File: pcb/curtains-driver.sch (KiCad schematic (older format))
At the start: 40 parts, among them J1 Barrel_Jack, J2 USB_B_Micro, J3 Motor, Q1 S8050, Q2 S8050, SW1 Reed_NC, SW2 Reed_NC, SW3 UP, SW4 DOWN, SW5 FLASH, SW6 RESET, U1 ESP-12F, U2 LM1117-3.3, U3 ULN2003, U4 CH340G, Y1 HC-49

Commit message: Update PCB
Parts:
- added R14: 10K, Resistor_SMD:R_0805_2012Metric_Pad1.15x1.40mm_HandSolder, symbol Device:R
- J1: symbol Connector:Barrel_Jack -> curtains-driver-rescue:Barrel_Jack-Connector
- SW5, SW6: footprint Button_Switch_SMD:SW_SPST_B3U-1000P -> Button_Switch_SMD:SW_SPST_TL3342
- U3: value ULN2003 -> ULN2003A
- Y1: footprint Crystal:Crystal_SMD_HC49-SD_HandSoldering -> Crystal:Crystal_SMD_SeikoEpson_FA238V-4Pin_3.2x2.5mm_HandSoldering; symbol Device:Crystal -> Device:Crystal_GND24_Small
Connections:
- wire segments 156 -> 159
- no-connect marks 20 -> 22
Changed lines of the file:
@@
 EESchema Schematic File Version 4
 LIBS:curtains-driver-cache
-EELAYER 26 0
+EELAYER 29 0
 EELAYER END
 $Descr A4 11693 8268
@@
 $EndComp
 $Comp
-L Connector:Barrel_Jack J1
+L curtains-driver-rescue:Barrel_Jack-Connector J1
 U 1 1 5C0D7D27
 P 5150 1750
@@
 P 9850 4250
 F 0 "U3" H 9850 4917 50  0000 C CNN
-F 1 "ULN2003" H 9850 4826 50  0000 C CNN
+F 1 "ULN2003A" H 9850 4826 50  0000 C CNN
 F 2 "Package_SO:SOIC-16W_5.3x10.2mm_P1.27mm" H 9900 3700 50  0001 L CNN
 F 3 "http://www.ti.com/lit/ds/symlink/uln2003a.pdf" H 9950 4050 50  0001 C CNN
@@
 F 0 "SW5" H 9500 5400 50  0000 L CNN
 F 1 "FLASH" H 9500 5300 50  0000 L CNN
-F 2 "Button_Switch_SMD:SW_SPST_B3U-1000P" H 9600 5150 50  0001 C CNN
+F 2 "Button_Switch_SMD:SW_SPST_TL3342" H 9600 5150 50  0001 C CNN
 F 3 "" H 9600 5150 50  0001 C CNN
 	1    9600 5150
@@
 	8700 5050 8700 5800
 Wire Wire Line
-	8950 3800 8950 4350
-Wire Wire Line
-	9050 3800 9050 4450
+	9050 3800 9050 4350
+Wire Wire Line
+	9150 3800 9150 4450
 $Comp
 L Switch:SW_SPST SW6
@@
 F 0 "SW6" H 6200 4000 50  0000 L CNN
 F 1 "RESET" H 6200 3900 50  0000 L CNN
-F 2 "Button_Switch_SMD:SW_SPST_B3U-1000P" H 6250 3750 50  0001 C CNN
+F 2 "Button_Switch_SMD:SW_SPST_TL3342" H 6250 3750 50  0001 C CNN
 F 3 "" H 6250 3750 50  0001 C CNN
 	1    6250 3750
@@
 	8650 4550 9450 4550
 Wire Wire Line
-	8650 4450 9050 4450
-Wire Wire Line
-	9050 4450 9450 4450
-Connection ~ 9050 4450
-Wire Wire Line
-	8650 4350 8950 4350
-Wire Wire Line
-	8950 4350 9450 4350
-Connection ~ 8950 4350
+	8650 4450 9150 4450
+Wire Wire Line
+	9150 4450 9450 4450
+Connection ~ 9150 4450
+Wire Wire Line
+	8650 4350 8800 4350
+Wire Wire Line
+	9050 4350 9450 4350
+Connection ~ 9050 4350
 Wire Wire Line
 	9850 5150 9850 4850
@@
 	1    0    0    -1
 $EndComp
-Text GLabel 8950 3800 1    50   Input ~ 0
+Text GLabel 9050 3800 1    50   Input ~ 0
 TXD
-Text GLabel 9050 3800 1    50   Input ~ 0
+Text GLabel 9150 3800 1    50   Input ~ 0
 RXD
 Text GLabel 3750 2950 2    50   Input ~ 0
@@
 	1750 3250 2500 3250
 $Comp
-L Device:Crystal Y1
+L Device:Crystal_GND24_Small Y1
 U 1 1 5C2E463A
 P 2200 3650
 F 0 "Y1" H 2200 3918 50  0000 C CNN
 F 1 "HC-49" H 2200 3827 50  0000 C CNN
-F 2 "Crystal:Crystal_SMD_HC49-SD_HandSoldering" H 2200 3650 50  0001 C CNN
+F 2 "Crystal:Crystal_SMD_SeikoEpson_FA238V-4Pin_3.2x2.5mm_HandSoldering" H 2200 3650 50  0001 C CNN
 F 3 "https://www.chipdip.ru/product/12mhz-hc-49sm" H 2200 3650 50  0001 C CNN
 	1    2200 3650
 	1    0    0    -1
 $EndComp
-Wire Wire Line
-	2350 3650 2400 3650
-Wire Wire Line
-	2050 3650 1900 3650
 Wire Wire Line
 	1900 3650 1900 3450
@@
 Wire Wire Line
 	3700 2950 3750 2950
+$Comp
+L Device:R R14
+U 1 1 5C37AADA
+P 8800 4100
+F 0 "R14" H 8600 4050 50  0000 L CNN
+F 1 "10K" H 8600 4150 50  0000 L CNN
+F 2 "Resistor_SMD:R_0805_2012Metric_Pad1.15x1.40mm_HandSolder" V 8730 4100 50  0001 C CNN
+F 3 "~" H 8800 4100 50  0001 C CNN
+	1    8800 4100
+	-1   0    0    1
+$EndComp
+Text GLabel 8800 3800 1    50   Input ~ 0
+VCC
+Wire Wire Line
+	8800 4250 8800 4350
+Connection ~ 8800 4350
+Wire Wire Line
+	8800 4350 9050 4350
+Wire Wire Line
+	8800 3800 8800 3950
+NoConn ~ 2200 3525
+Wire Wire Line
+	1900 3650 2100 3650
+Wire Wire Line
+	2300 3650 2400 3650
+NoConn ~ 2200 3775
 $EndSCHEMATC

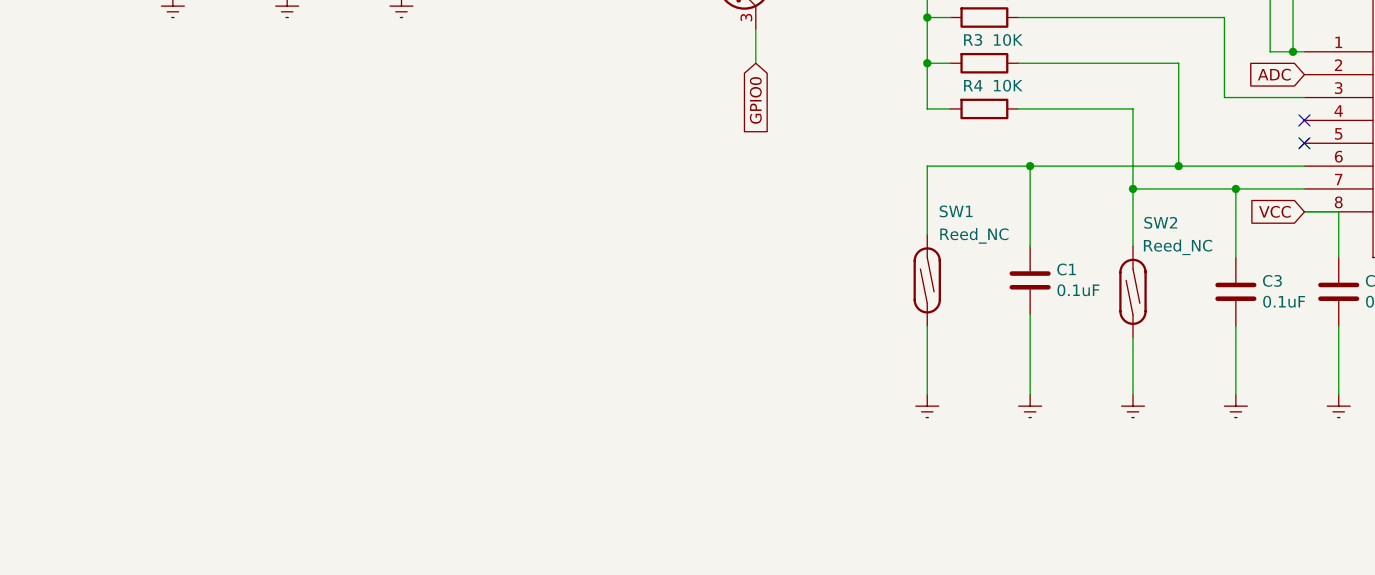
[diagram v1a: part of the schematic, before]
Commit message: Minimal working result
Signed-off-by: Mikhail Baranov <mikhail.baranov@gmail.com>
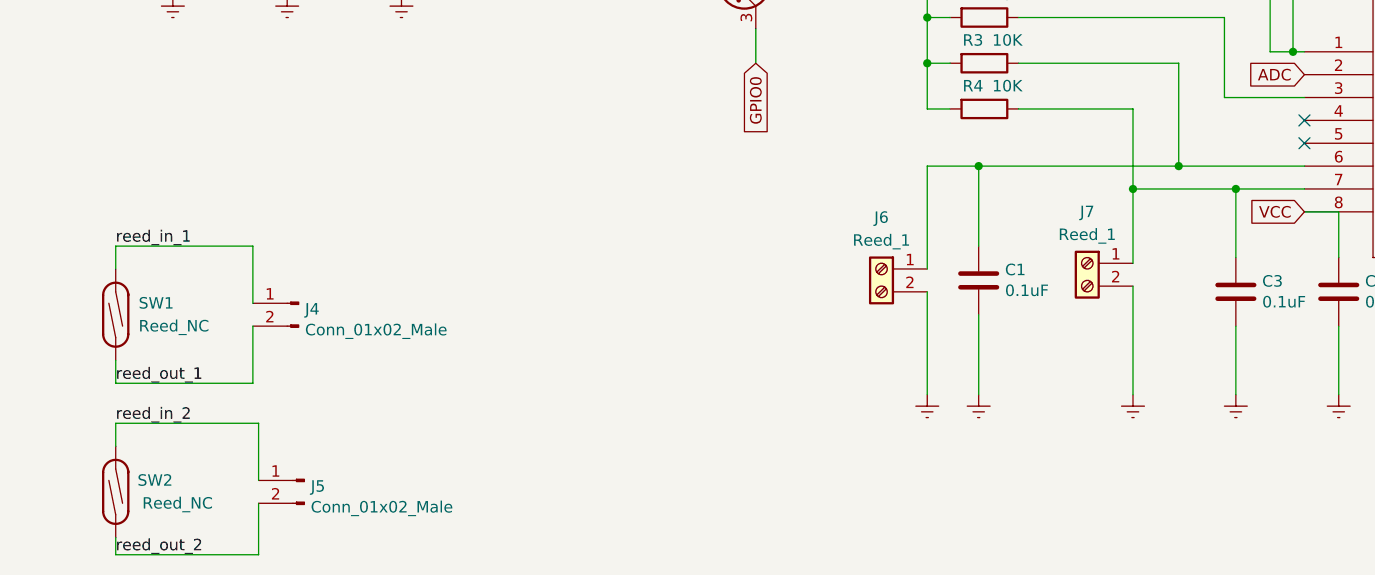
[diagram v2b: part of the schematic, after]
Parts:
- added J4, J5: Conn_01x02_Male, Connector_PinHeader_2.54mm:PinHeader_1x02_P2.54mm_Horizontal, symbol Connector:Conn_01x02_Male
- added J6, J7: Reed_1, TerminalBlock_TE-Connectivity:TerminalBlock_TE_282834-2_1x02_P2.54mm_Horizontal, symbol Connector:Screw_Terminal_01x02
- SW1, SW2: footprint TerminalBlock_TE-Connectivity:TerminalBlock_TE_282834-2_1x02_P2.54mm_Horizontal -> Resistor_THT:R_Axial_Power_L20.0mm_W6.4mm_P30.48mm
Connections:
- net Earth: now also J6.2 (Pin_2), J7.2 (Pin_2); no longer SW1.1, SW2.1
- net at C1.1, R3.1, U1.6 (GPIO12): now also J6.1 (Pin_1); no longer SW1.2
- net at C3.1, R4.1, U1.7 (GPIO13): now also J7.1 (Pin_1); no longer SW2.2
- new net reed_in_1: J4.1 (Pin_1), SW1.2
- new net reed_in_2: J5.1 (Pin_1), SW2.2
- new net reed_out_1: J4.2 (Pin_2), SW1.1
- new net reed_out_2: J5.2 (Pin_2), SW2.1
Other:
- moved on the sheet: C1, SW1, SW2
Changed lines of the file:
@@
 L Switch:SW_Reed SW1
 U 1 1 5C0D94BB
-P 5200 5350
-F 0 "SW1" V 5500 5300 50  0000 R CNN
-F 1 "Reed_NC" V 5400 5300 50  0000 R CNN
-F 2 "TerminalBlock_TE-Connectivity:TerminalBlock_TE_282834-2_1x02_P2.54mm_Horizontal" H 5200 5350 50  0001 C CNN
-F 3 "" H 5200 5350 50  0001 C CNN
-	1    5200 5350
+P 1650 5500
+F 0 "SW1" V 1700 5400 50  0000 R CNN
+F 1 "Reed_NC" V 1600 5400 50  0000 R CNN
+F 2 "Resistor_THT:R_Axial_Power_L20.0mm_W6.4mm_P30.48mm" H 1650 5500 50  0001 C CNN
+F 3 "" H 1650 5500 50  0001 C CNN
+	1    1650 5500
 	0    -1   -1   0
 $EndComp
@@
 L Switch:SW_Reed SW2
 U 1 1 5C0D9634
-P 6100 5400
-F 0 "SW2" V 6400 5200 50  0000 L CNN
-F 1 "Reed_NC" V 6300 5050 50  0000 L CNN
-F 2 "TerminalBlock_TE-Connectivity:TerminalBlock_TE_282834-2_1x02_P2.54mm_Horizontal" H 6100 5400 50  0001 C CNN
-F 3 "" H 6100 5400 50  0001 C CNN
-	1    6100 5400
+P 1650 6275
+F 0 "SW2" V 1700 6025 50  0000 L CNN
+F 1 "Reed_NC" V 1600 5850 50  0000 L CNN
+F 2 "Resistor_THT:R_Axial_Power_L20.0mm_W6.4mm_P30.48mm" H 1650 6275 50  0001 C CNN
+F 3 "" H 1650 6275 50  0001 C CNN
+	1    1650 6275
 	0    -1   -1   0
 $EndComp
@@
 NoConn ~ 7900 5550
 NoConn ~ 8000 5550
-Wire Wire Line
-	6100 4950 6100 5200
 $Comp
 L power:Earth #PWR0107
@@
 	1    0    0    -1
 $EndComp
-Wire Wire Line
-	6100 5600 6100 5850
-Wire Wire Line
-	5200 5550 5200 5850
 $Comp
 L Device:C C2
@@
 L Device:C C1
 U 1 1 5C14C6AA
-P 5650 5350
-F 0 "C1" H 5765 5396 50  0000 L CNN
-F 1 "0.1uF" H 5765 5305 50  0000 L CNN
-F 2 "Capacitor_SMD:C_1206_3216Metric_Pad1.42x1.75mm_HandSolder" H 5688 5200 50  0001 C CNN
-F 3 "~" H 5650 5350 50  0001 C CNN
-	1    5650 5350
+P 5425 5350
+F 0 "C1" H 5540 5396 50  0000 L CNN
+F 1 "0.1uF" H 5540 5305 50  0000 L CNN
+F 2 "Capacitor_SMD:C_1206_3216Metric_Pad1.42x1.75mm_HandSolder" H 5463 5200 50  0001 C CNN
+F 3 "~" H 5425 5350 50  0001 C CNN
+	1    5425 5350
 	1    0    0    -1
 $EndComp
@@
 L power:Earth #PWR0115
 U 1 1 5C152829
-P 5650 5850
-F 0 "#PWR0115" H 5650 5600 50  0001 C CNN
-F 1 "Earth" H 5650 5700 50  0001 C CNN
-F 2 "" H 5650 5850 50  0001 C CNN
-F 3 "~" H 5650 5850 50  0001 C CNN
-	1    5650 5850
-	1    0    0    -1
-$EndComp
-Wire Wire Line
-	5650 5500 5650 5850
+P 5425 5850
+F 0 "#PWR0115" H 5425 5600 50  0001 C CNN
+F 1 "Earth" H 5425 5700 50  0001 C CNN
+F 2 "" H 5425 5850 50  0001 C CNN
+F 3 "~" H 5425 5850 50  0001 C CNN
+	1    5425 5850
+	1    0    0    -1
+$EndComp
+Wire Wire Line
+	5425 5500 5425 5850
 Wire Wire Line
 	6550 5550 6550 5850
@@
 	8950 2250 9400 2250
 Wire Wire Line
-	5200 4850 5200 5150
-Wire Wire Line
-	5650 4850 5650 5200
+	5425 4850 5425 5200
 $Comp
 L power:+3.3V #PWR0109
@@
 $EndComp
 Wire Wire Line
-	5200 4850 5650 4850
-Connection ~ 5650 4850
+	5200 4850 5425 4850
+Connection ~ 5425 4850
 Wire Wire Line
 	6100 4950 6550 4950
@@
 	6300 4850 6300 4400
 Wire Wire Line
-	5650 4850 6300 4850
+	5425 4850 6300 4850
 Connection ~ 6300 4850
 Wire Wire Line
@@
 	2300 3650 2400 3650
 NoConn ~ 2200 3775
+$Comp
+L Connector:Screw_Terminal_01x02 J6
+U 1 1 5CABFAC7
+P 5000 5300
+F 0 "J6" H 5000 5525 50  0000 C CNN
+F 1 "Reed_1" H 5000 5425 50  0000 C CNN
+F 2 "TerminalBlock_TE-Connectivity:TerminalBlock_TE_282834-2_1x02_P2.54mm_Horizontal" H 5000 5300 50  0001 C CNN
+F 3 "~" H 5000 5300 50  0001 C CNN
+	1    5000 5300
+	-1   0    0    -1
+$EndComp
+Wire Wire Line
+	5200 4850 5200 5300
+Wire Wire Line
+	5200 5400 5200 5850
+$Comp
+L Connector:Screw_Terminal_01x02 J7
+U 1 1 5CAF933C
+P 5900 5275
+F 0 "J7" H 5900 5500 50  0000 C CNN
+F 1 "Reed_1" H 5900 5400 50  0000 C CNN
+F 2 "TerminalBlock_TE-Connectivity:TerminalBlock_TE_282834-2_1x02_P2.54mm_Horizontal" H 5900 5275 50  0001 C CNN
+F 3 "~" H 5900 5275 50  0001 C CNN
+	1    5900 5275
+	-1   0    0    -1
+$EndComp
+Wire Wire Line
+	6100 4950 6100 5275
+Wire Wire Line
+	6100 5375 6100 5850
+$Comp
+L Connector:Conn_01x02_Male J4
+U 1 1 5CB2C5B6
+P 2450 5450
+F 0 "J4" H 2422 5424 50  0000 R CNN
+F 1 "Conn_01x02_Male" H 2422 5333 50  0000 R CNN
+F 2 "Connector_PinHeader_2.54mm:PinHeader_1x02_P2.54mm_Horizontal" H 2450 5450 50  0001 C CNN
+F 3 "~" H 2450 5450 50  0001 C CNN
+	1    2450 5450
+	-1   0    0    -1
+$EndComp
+$Comp
+L Connector:Conn_01x02_Male J5
+U 1 1 5CB348F6
+P 2475 6225
+F 0 "J5" H 2447 6199 50  0000 R CNN
+F 1 "Conn_01x02_Male" H 2447 6108 50  0000 R CNN
+F 2 "Connector_PinHeader_2.54mm:PinHeader_1x02_P2.54mm_Horizontal" H 2475 6225 50  0001 C CNN
+F 3 "~" H 2475 6225 50  0001 C CNN
+	1    2475 6225
+	-1   0    0    -1
+$EndComp
+Wire Wire Line
+	1650 5300 1650 5200
+Wire Wire Line
+	1650 5200 2250 5200
+Wire Wire Line
+	2250 5200 2250 5450
+Wire Wire Line
+	1650 5700 1650 5800
+Wire Wire Line
+	1650 5800 2250 5800
+Wire Wire Line
+	2250 5800 2250 5550
+Wire Wire Line
+	1650 6075 1650 5975
+Wire Wire Line
+	1650 5975 2275 5975
+Wire Wire Line
+	2275 5975 2275 6225
+Wire Wire Line
+	1650 6475 1650 6550
+Wire Wire Line
+	1650 6550 2275 6550
+Wire Wire Line
+	2275 6550 2275 6325
+Text Label 1650 5200 0    50   ~ 0
+reed_in_1
+Text Label 1650 5800 0    50   ~ 0
+reed_out_1
+Text Label 1650 5975 0    50   ~ 0
+reed_in_2
+Text Label 1650 6550 0    50   ~ 0
+reed_out_2
 $EndSCHEMATC
